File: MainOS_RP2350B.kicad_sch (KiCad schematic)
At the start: 12 parts, among them U4 RP2350B-QFN80, Y1 12 MHz

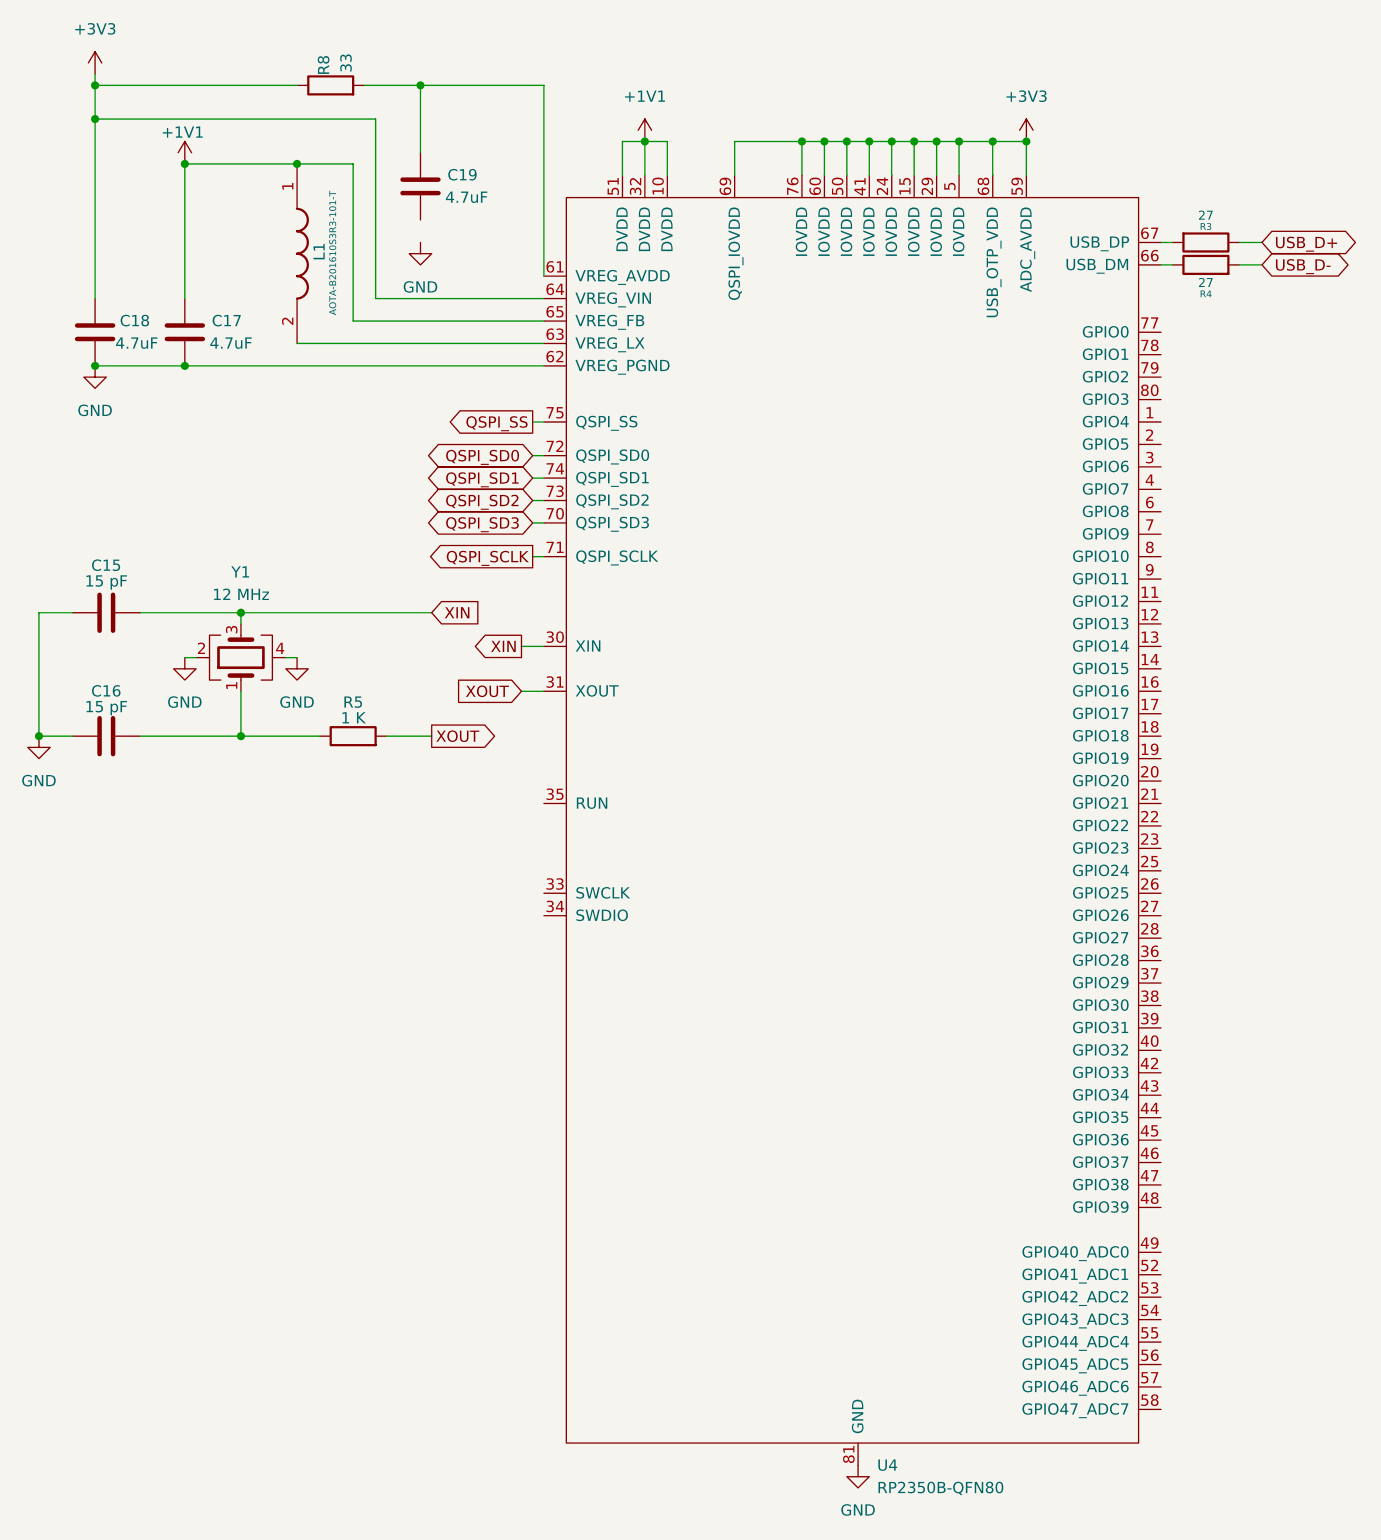
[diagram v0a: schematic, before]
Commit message: Restore Local Backup
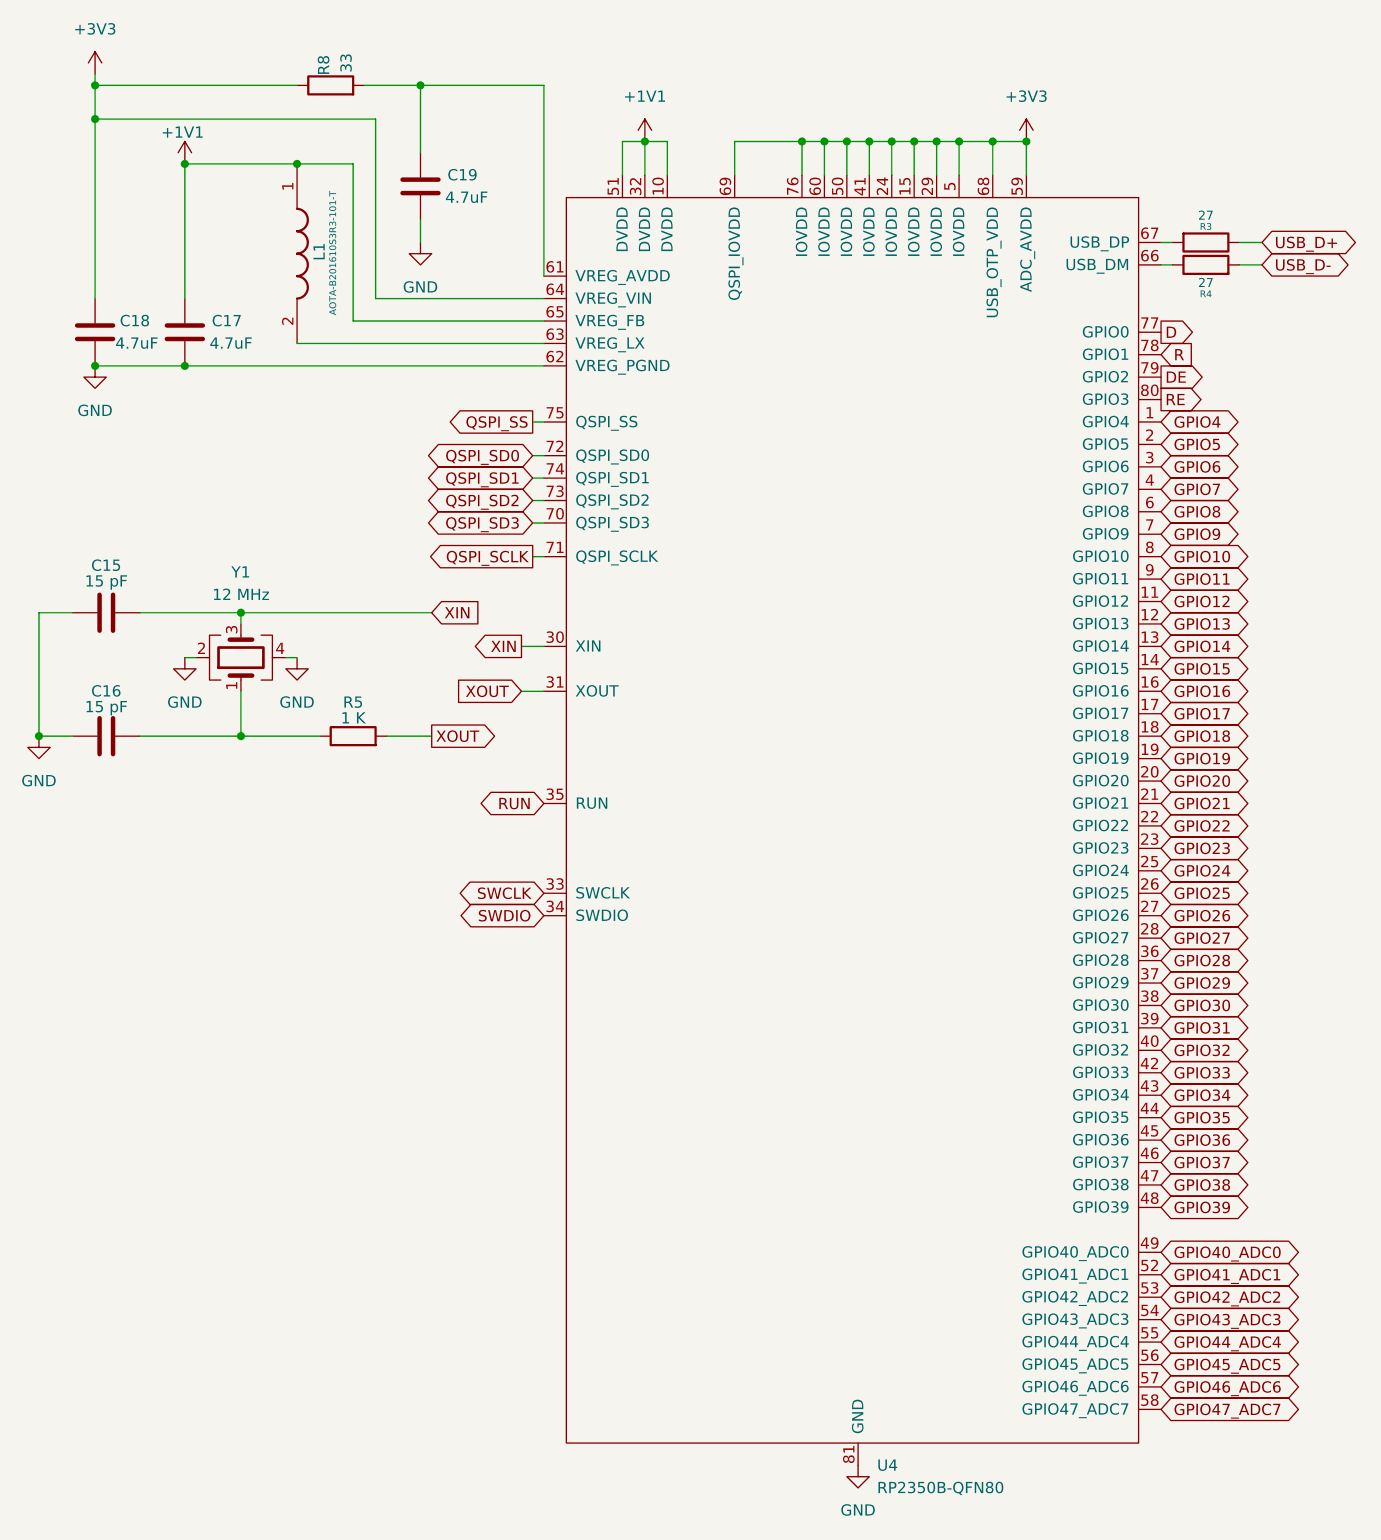
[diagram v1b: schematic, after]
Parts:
- C15, C16, C17, C18, C19: footprint (none) -> Capacitor_SMD:C_0402_1005Metric
- L1: footprint AOTAB201610S3R3101T -> JonasLib-Git:AOTAB201610S3R3101T
- R3, R4, R5, R8: footprint (none) -> Resistor_SMD:R_0402_1005Metric
- U4: footprint (none) -> Package_DFN_QFN:QFN-80-1EP_10x10mm_P0.4mm_EP3.4x3.4mm
- Y1: footprint (none) -> Crystal:Crystal_SMD_3225-4Pin_3.2x2.5mm
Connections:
- net GND: now also C19.2
- net GPIO4: now reaches U4.1 (GPIO4)
- net GPIO12: now reaches U4.11 (GPIO12)
- net GPIO13: now reaches U4.12 (GPIO13)
- net GPIO14: now reaches U4.13 (GPIO14)
- net GPIO15: now reaches U4.14 (GPIO15)
- net GPIO16: now reaches U4.16 (GPIO16)
- net GPIO17: now reaches U4.17 (GPIO17)
- net GPIO18: now reaches U4.18 (GPIO18)
- net GPIO19: now reaches U4.19 (GPIO19)
- net GPIO5: now reaches U4.2 (GPIO5)
- net GPIO20: now reaches U4.20 (GPIO20)
- net GPIO21: now reaches U4.21 (GPIO21)
- net GPIO22: now reaches U4.22 (GPIO22)
- net GPIO23: now reaches U4.23 (GPIO23)
- net GPIO24: now reaches U4.25 (GPIO24)
- net GPIO25: now reaches U4.26 (GPIO25)
- net GPIO26: now reaches U4.27 (GPIO26)
- net GPIO27: now reaches U4.28 (GPIO27)
- net GPIO6: now reaches U4.3 (GPIO6)
- net SWCLK: now reaches U4.33 (SWCLK)
- net SWDIO: now reaches U4.34 (SWDIO)
- net RUN: now reaches U4.35 (RUN)
- net GPIO28: now reaches U4.36 (GPIO28)
- net GPIO29: now reaches U4.37 (GPIO29)
- net GPIO30: now reaches U4.38 (GPIO30)
- net GPIO31: now reaches U4.39 (GPIO31)
- net GPIO7: now reaches U4.4 (GPIO7)
- net GPIO32: now reaches U4.40 (GPIO32)
- net GPIO33: now reaches U4.42 (GPIO33)
- net GPIO34: now reaches U4.43 (GPIO34)
- net GPIO35: now reaches U4.44 (GPIO35)
- net GPIO36: now reaches U4.45 (GPIO36)
- net GPIO37: now reaches U4.46 (GPIO37)
- net GPIO38: now reaches U4.47 (GPIO38)
- net GPIO39: now reaches U4.48 (GPIO39)
- net GPIO40_ADC0: now reaches U4.49 (GPIO40_ADC0)
- net GPIO41_ADC1: now reaches U4.52 (GPIO41_ADC1)
- net GPIO42_ADC2: now reaches U4.53 (GPIO42_ADC2)
- net GPIO43_ADC3: now reaches U4.54 (GPIO43_ADC3)
- net GPIO44_ADC4: now reaches U4.55 (GPIO44_ADC4)
- net GPIO45_ADC5: now reaches U4.56 (GPIO45_ADC5)
- net GPIO46_ADC6: now reaches U4.57 (GPIO46_ADC6)
- net GPIO47_ADC7: now reaches U4.58 (GPIO47_ADC7)
- net GPIO8: now reaches U4.6 (GPIO8)
- net GPIO9: now reaches U4.7 (GPIO9)
- net D: now reaches U4.77 (GPIO0)
- net R: now reaches U4.78 (GPIO1)
- net DE: now reaches U4.79 (GPIO2)
- net GPIO10: now reaches U4.8 (GPIO10)
- net RE: now reaches U4.80 (GPIO3)
- net GPIO11: now reaches U4.9 (GPIO11)
